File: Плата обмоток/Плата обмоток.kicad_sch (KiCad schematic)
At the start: 22 parts, among them J1 4900, J10 4900, J11 4900, J12 4900, J13 4900, J14 A1, J15 A2, J16 B1, J17 B2, J18 C1, J19 C2, J2 4900, J3 4900, J4 Conn_01x02, J6 Conn_01x02, J7 Conn_01x02, J8 4900, J8 Conn_02x02_Odd_Even, J9 4900

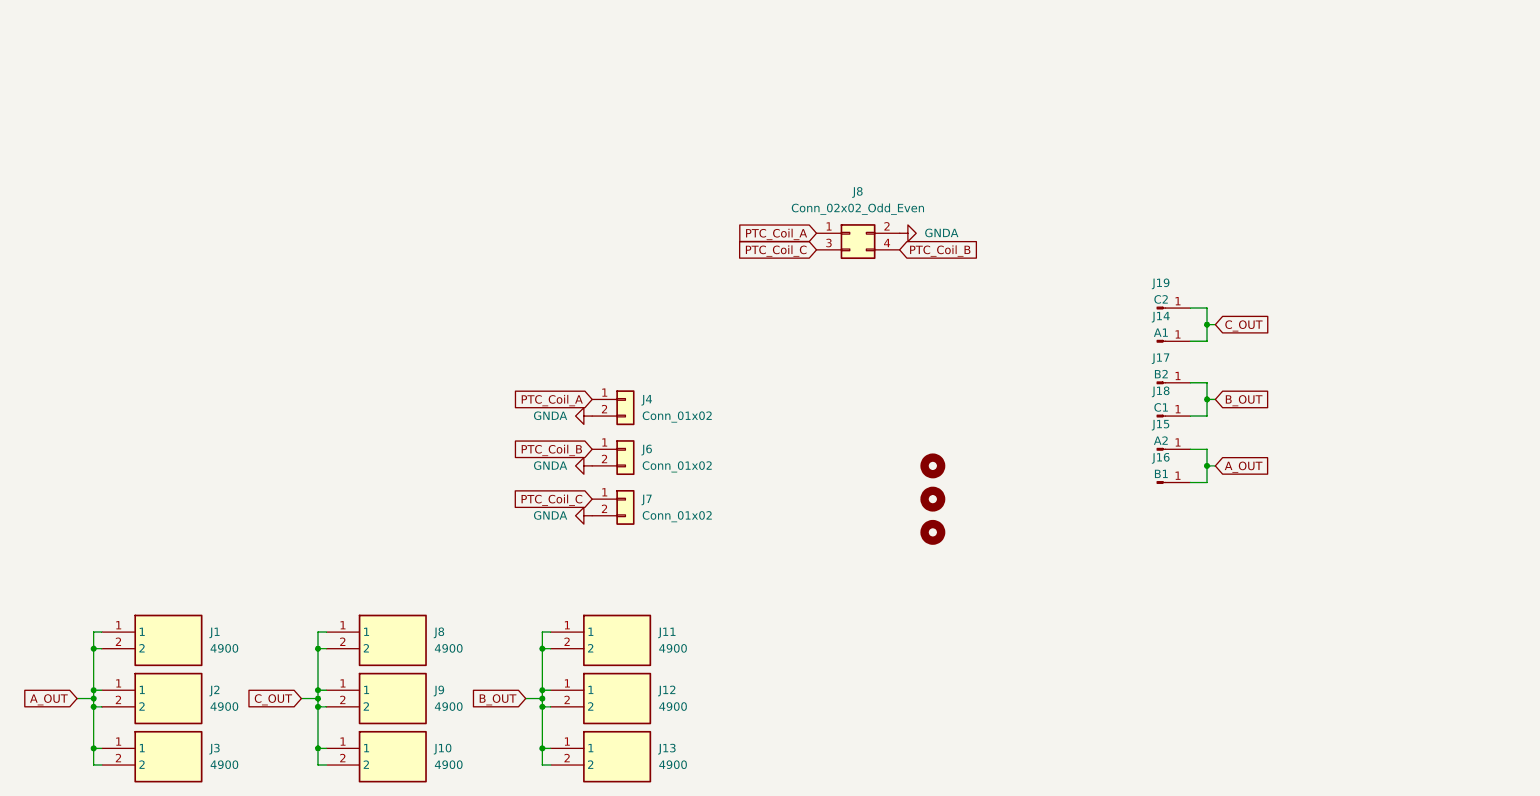
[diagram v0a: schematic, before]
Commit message: Добавил все документы
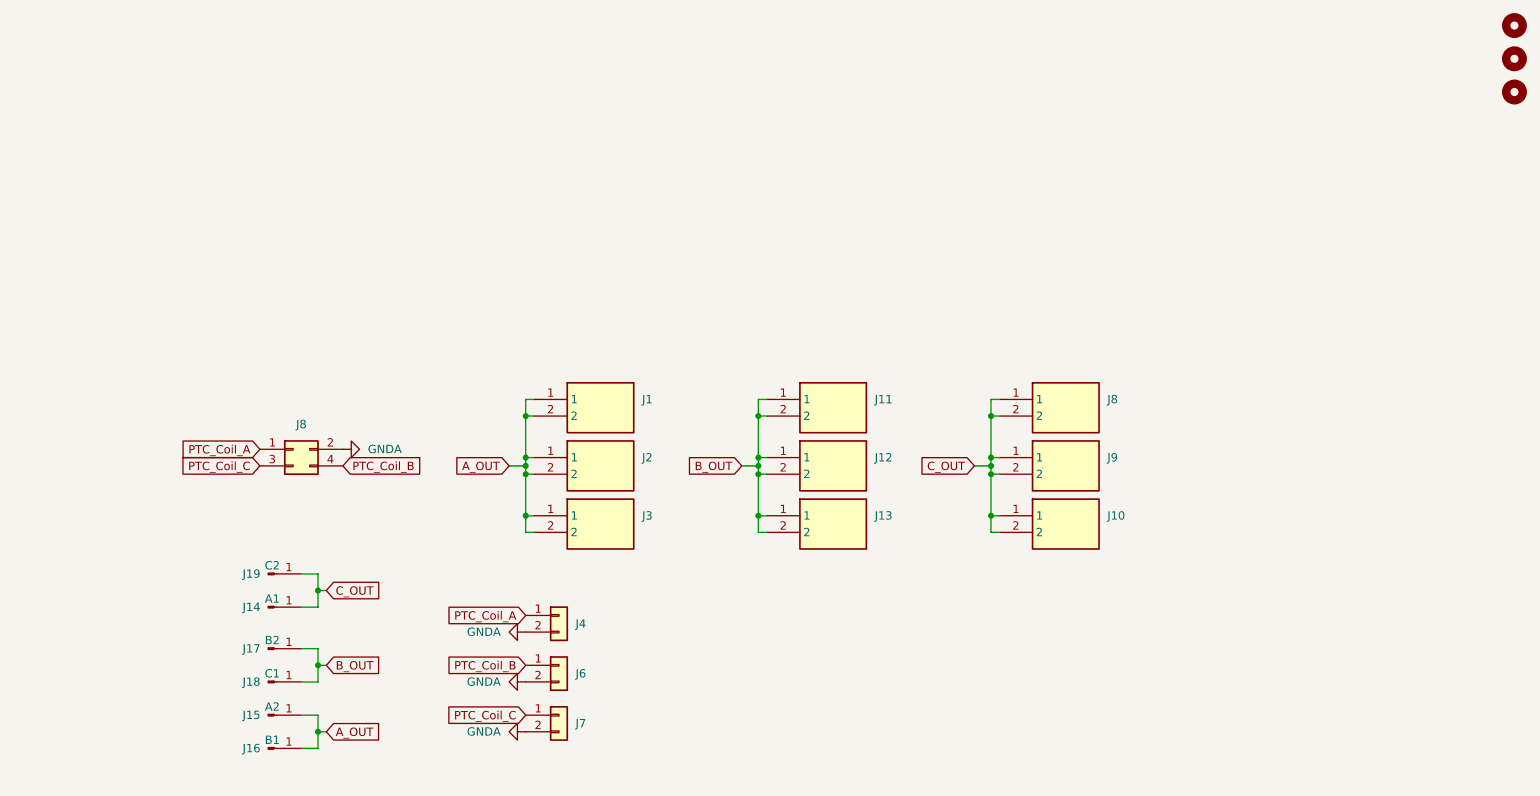
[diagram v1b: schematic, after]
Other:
- title: (none) -> Соединительная плата ЭЛП
- moved on the sheet: J1, J10, J11, J12, J13, J14, J15, J16, J17, J18, J19, J2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
